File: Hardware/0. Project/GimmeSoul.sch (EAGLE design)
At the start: 15 parts, among them U2 ATMEGA328P-AU

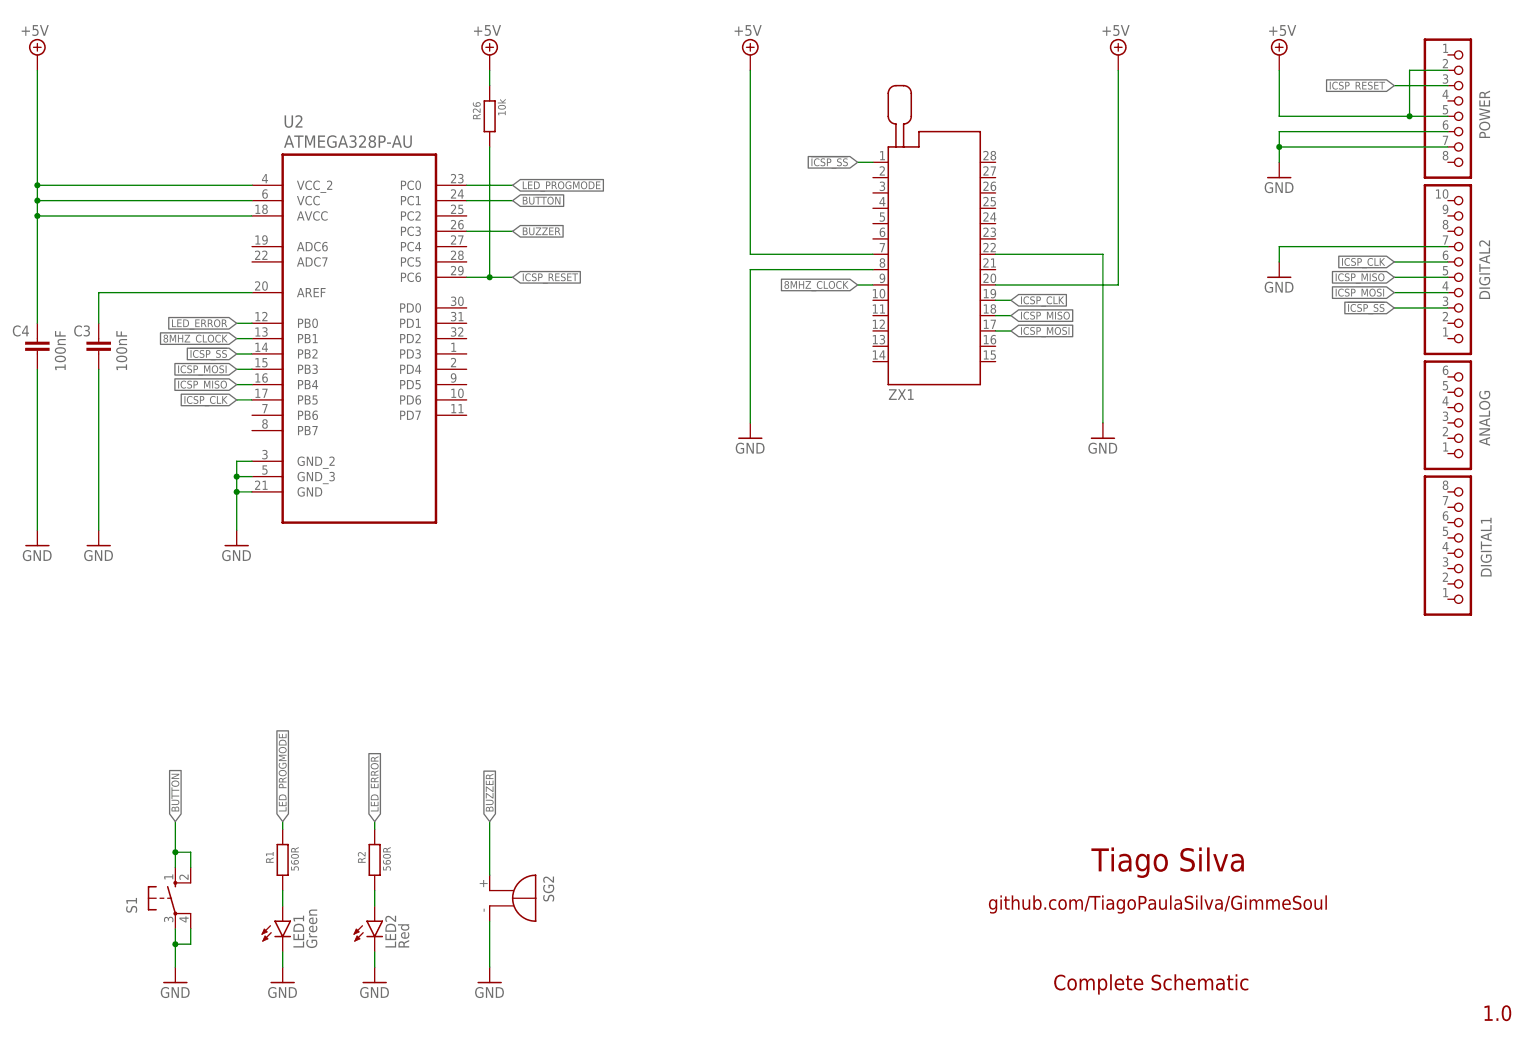
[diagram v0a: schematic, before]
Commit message: Schematic minor improvements
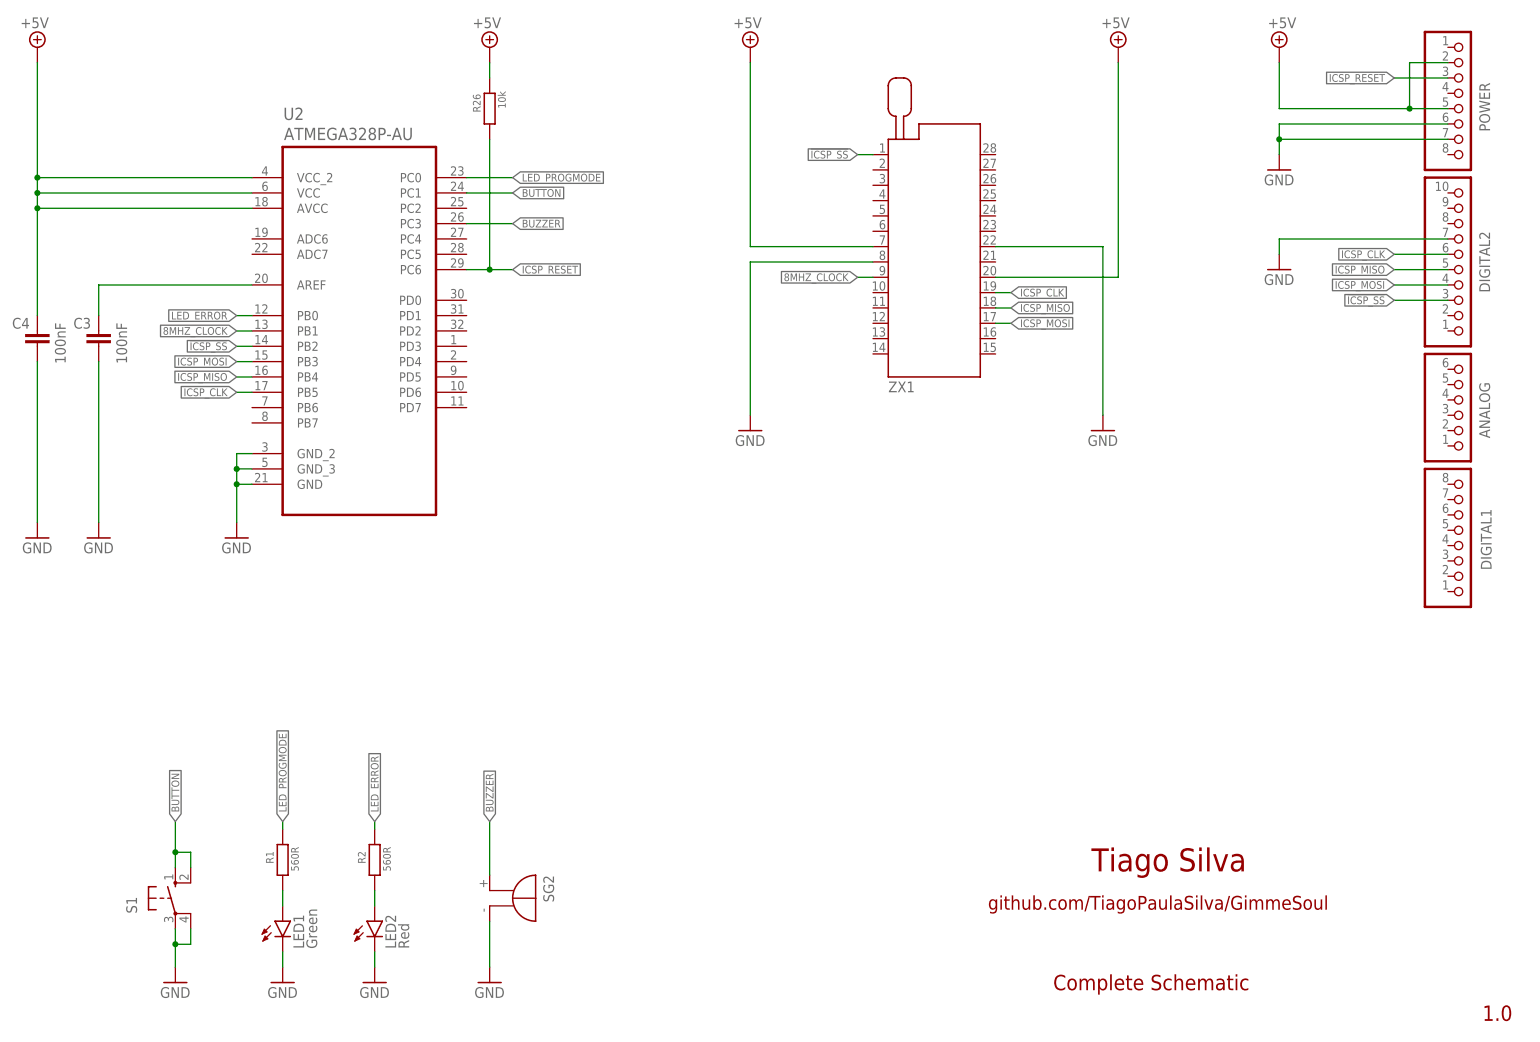
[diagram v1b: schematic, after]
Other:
- note removed: "POWER SUPPLY & BATTERY STATUS MONITOR"
- moved on the sheet: ANALOG, C3, C4, DIGITAL1, DIGITAL2, POWER, R26, U2, ZX1
